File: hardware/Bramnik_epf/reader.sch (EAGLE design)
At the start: 8 parts, among them X1 RJ11

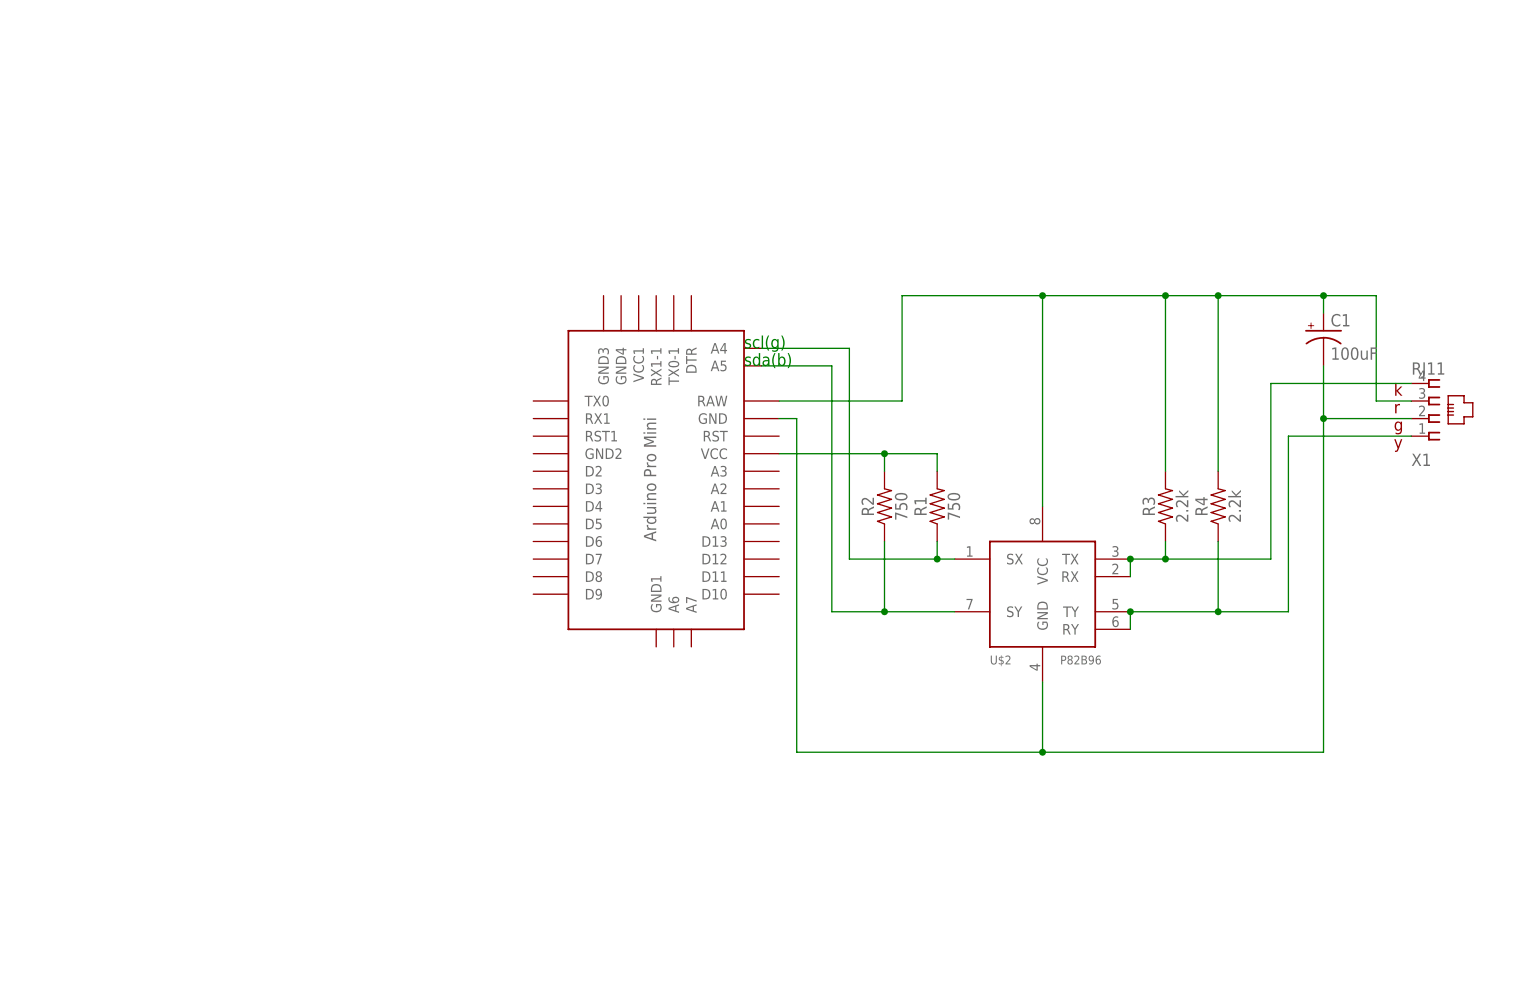
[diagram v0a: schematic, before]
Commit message: Upd scheme
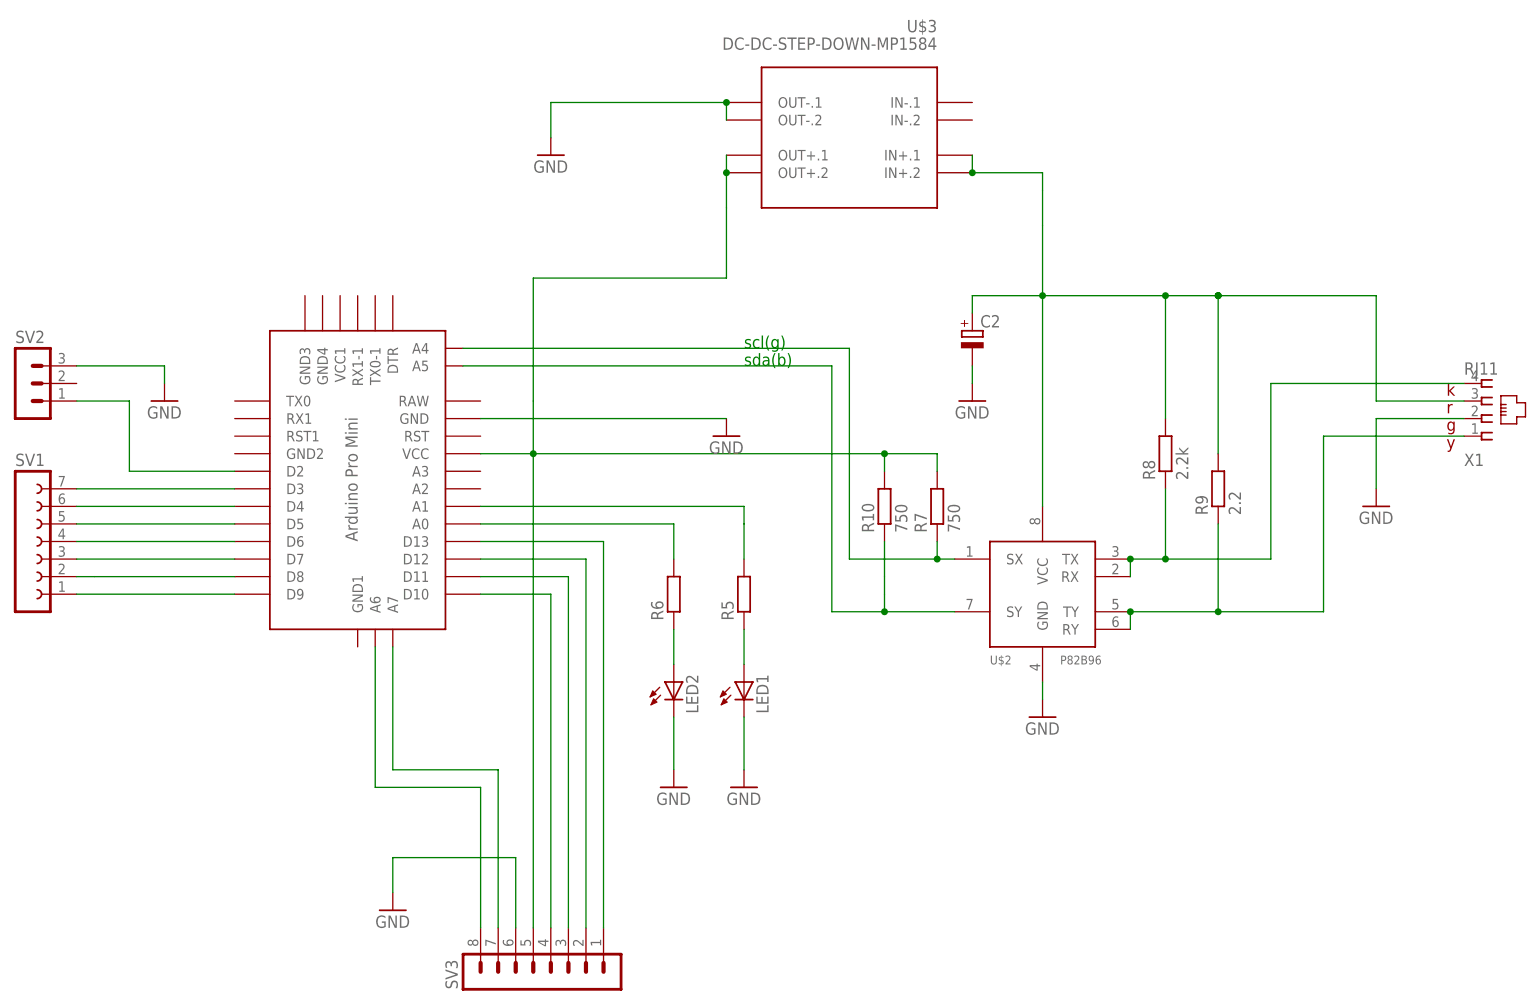
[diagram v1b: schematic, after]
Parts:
- removed C1: 100uF, SparkFun-Capacitors:100UF-POLAR-10X10.5-63V-20%
- removed R1, R2: 750, SparkFun-Resistors:750OHM-0603-1/10W-1%
- removed R3, R4: 2.2k, SparkFun-Resistors:2.2KOHM-0603-1/10W-1%
- added C2: (no value), rcl:CPOL-EUE5-6
- added LED1, LED2: (no value), led:LEDB152
- added R10, R7: 750, rcl:R-EU_M1206
- added R5, R6: (no value), rcl:R-EU_M1206
- added R8: 2.2k, rcl:R-EU_M1206
- added R9: 2.2, rcl:R-EU_M1206
- added SV1: (no value), con-lsta:FE07-1
- added SV2: (no value), con-lstb:MA03-1
- added SV3: (no value), con-lstb:MA08-1
- added U$3: DC-DC-STEP-DOWN-MP1584, diy-modules:DC-DC-STEP-DOWN-MP1584
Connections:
- removed net N$2: R1.2, R2.2, U$1.VCC
- new net GND: C2.-, LED1.C, LED2.C, SV2.3, SV3.6, U$1.GND, U$2.GND, U$3.OUT-.1, U$3.OUT-.2, X1.2
- new net N$1: SV1.1, U$1.D9
- new net N$10: SV1.3, U$1.D7
- new net N$11: SV1.4, U$1.D6
- new net N$12: SV1.5, U$1.D5
- new net N$13: SV1.6, U$1.D4
- new net N$14: SV1.7, U$1.D3
- new net N$15: SV3.2, U$1.D12
- new net N$16: SV2.1, U$1.D2
- new net N$17: R5.2, U$1.A1
- new net N$18: R6.2, U$1.A0
- new net N$19: LED1.A, R5.1
- new net N$20: LED2.A, R6.1
- new net N$21: SV3.3, U$1.D11
- new net N$22: R10.2, R7.2, SV3.5, U$1.VCC, U$3.OUT+.1, U$3.OUT+.2
- new net N$23: SV3.4, U$1.D10
- new net N$24: SV3.7, U$1.A7
- new net N$25: SV3.8, U$1.A6
- new net N$8: SV1.2, U$1.D8
- net N$3: now also R7.1; no longer R1.1
- net N$4: now also R10.1; no longer R2.1
- net N$5: now also R8.1; no longer R3.1
- net N$6: now also SV3.1, U$1.D13; no longer C1.-, U$1.GND, U$2.GND, X1.2
- net N$7: now also R9.1; no longer R4.1
- net N$9: now also C2.+, R8.2, R9.2, U$3.IN+.1, U$3.IN+.2; no longer C1.+, R3.2, R4.2, U$1.RAW
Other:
- moved on the sheet: X1
